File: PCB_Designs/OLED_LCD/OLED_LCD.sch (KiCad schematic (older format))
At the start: 27 parts, among them P1 CONN_01X10, P2 CONN_01X16, P3 CONN_01X01, P4 CONN_01X01, P5 CONN_01X01, P6 CONN_01X01, SW1 Rotary_Encoder_Switch, U2 MCP23017, U3 CHERRY-MX

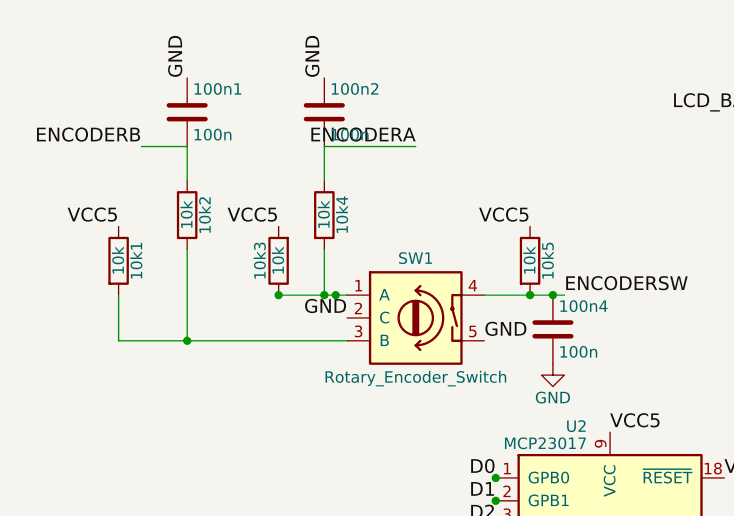
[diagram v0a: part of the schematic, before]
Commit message: New stuff
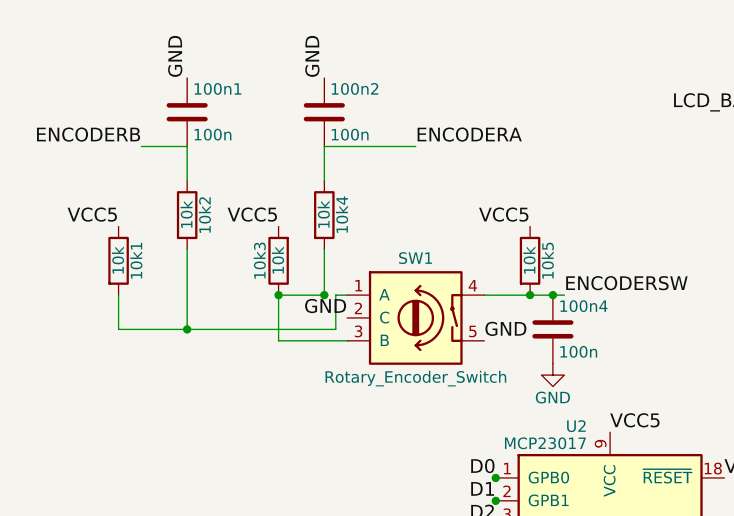
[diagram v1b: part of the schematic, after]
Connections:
- net at 10k3.1, 10k4.2: now also SW1.3 (B); no longer SW1.1 (A)
- net at 10k1.2, 10k2.2: now also SW1.1 (A); no longer SW1.3 (B)
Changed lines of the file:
@@
 	1    0    0    -1
 $EndComp
-Text Label 3700 1100 2    60   ~ 0
+Text Label 3700 1100 0    60   ~ 0
 ENCODERA
 Text Label 2500 1100 2    60   ~ 0
@@
 	2500 1100 2700 1100
 Wire Wire Line
-	2400 1750 2400 1950
-Wire Wire Line
-	2400 1950 3400 1950
+	2400 1750 2400 1900
 Text Label 3400 1850 2    60   ~ 0
 GND
@@
 GND
 Connection ~ 3100 1750
-Connection ~ 3350 1750
-Connection ~ 2700 1950
+Connection ~ 2700 1900
 Text Label 3300 800  1    60   ~ 0
 GND
@@
 Connection ~ 3300 1750
 Wire Wire Line
-	2700 1550 2700 1950
+	2700 1550 2700 1900
 Wire Wire Line
 	3300 1100 3300 1250
@@
 Text Label 5800 1650 2    60   ~ 0
 INTA
-Wire Wire Line
-	3100 1750 3400 1750
 $Comp
 L C 100n4
@@
 	1    0    0    -1
 $EndComp
+Wire Wire Line
+	3300 1750 3100 1750
+Wire Wire Line
+	3100 1750 3100 1950
+Wire Wire Line
+	3100 1950 3400 1950
+Wire Wire Line
+	3400 1750 3350 1750
+Wire Wire Line
+	3350 1900 3350 1750
+Wire Wire Line
+	2400 1900 3350 1900
 $EndSCHEMATC
